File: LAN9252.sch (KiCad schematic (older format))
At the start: 52 parts, among them U1 LAN9252, U2 24LC00, Y1 Crystal_GND24

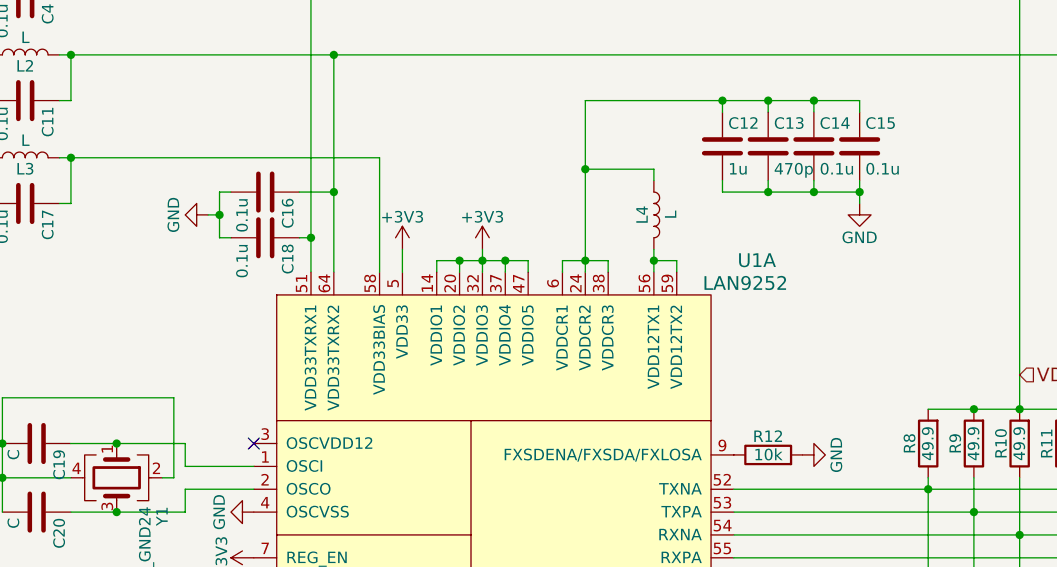
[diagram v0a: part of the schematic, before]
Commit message: 進捗
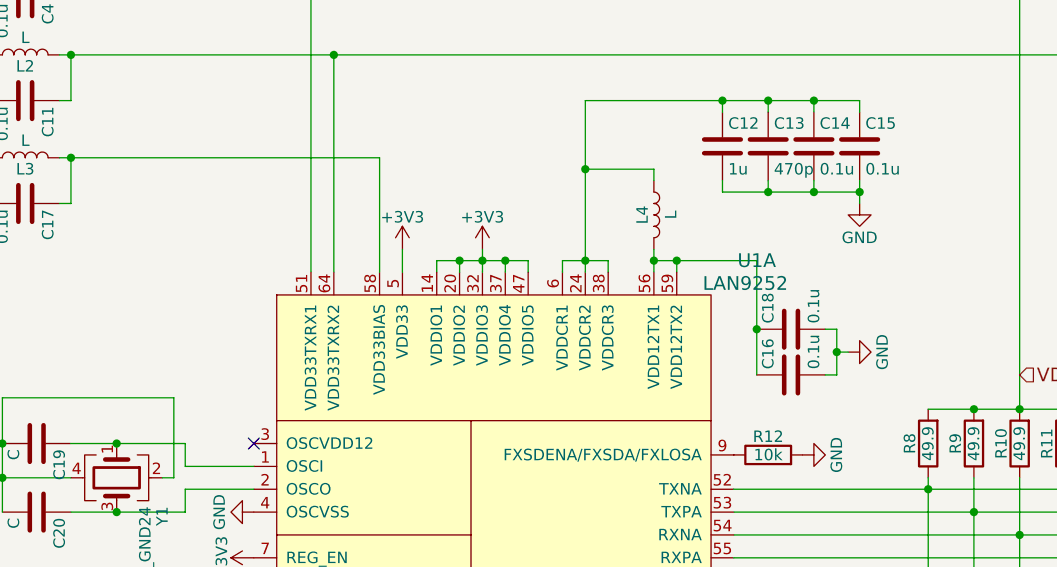
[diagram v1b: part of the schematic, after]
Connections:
- net VDD33TXRX1: no longer C18.1
- net VDDTXRX2: no longer C16.1
- net at L4.2, U1.56 (VDD12TX1), U1.59 (VDD12TX2): now also C16.1, C18.1
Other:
- moved on the sheet: C16, C18
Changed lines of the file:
@@
 $EndDescr
 $Comp
-L GND #PWR46
+L GND #PWR022
 U 1 1 58D8F4AE
 P 6400 6000
-F 0 "#PWR46" H 6400 5750 50  0001 C CNN
+F 0 "#PWR022" H 6400 5750 50  0001 C CNN
 F 1 "GND" H 6400 5850 50  0000 C CNN
 F 2 "" H 6400 6000 50  0000 C CNN
@@
 NoConn ~ 4600 3850
 $Comp
-L GND #PWR32
+L GND #PWR023
 U 1 1 58D8FBF8
 P 4600 4150
-F 0 "#PWR32" H 4600 3900 50  0001 C CNN
+F 0 "#PWR023" H 4600 3900 50  0001 C CNN
 F 1 "GND" H 4600 4000 50  0000 C CNN
 F 2 "" H 4600 4150 50  0000 C CNN
@@
 $EndComp
 $Comp
-L GND #PWR34
+L GND #PWR024
 U 1 1 58D8FC8D
 P 4250 4500
-F 0 "#PWR34" H 4250 4250 50  0001 C CNN
+F 0 "#PWR024" H 4250 4250 50  0001 C CNN
 F 1 "GND" H 4250 4350 50  0000 C CNN
 F 2 "" H 4250 4500 50  0000 C CNN
@@
 $EndComp
 $Comp
-L GND #PWR40
+L GND #PWR025
 U 1 1 58D8FD81
 P 4600 5100
-F 0 "#PWR40" H 4600 4850 50  0001 C CNN
+F 0 "#PWR025" H 4600 4850 50  0001 C CNN
 F 1 "GND" H 4600 4950 50  0000 C CNN
 F 2 "" H 4600 5100 50  0000 C CNN
@@
 $EndComp
 $Comp
-L GND #PWR30
+L GND #PWR026
 U 1 1 58D8CF70
 P 7000 3900
-F 0 "#PWR30" H 7000 3650 50  0001 C CNN
+F 0 "#PWR026" H 7000 3650 50  0001 C CNN
 F 1 "GND" H 7000 3750 50  0000 C CNN
 F 2 "" H 7000 3900 50  0000 C CNN
@@
 $EndComp
 $Comp
-L GND #PWR41
+L GND #PWR027
 U 1 1 58D8D10E
 P 7000 5350
-F 0 "#PWR41" H 7000 5100 50  0001 C CNN
+F 0 "#PWR027" H 7000 5100 50  0001 C CNN
 F 1 "GND" H 7000 5200 50  0000 C CNN
 F 2 "" H 7000 5350 50  0000 C CNN
@@
 $EndComp
 $Comp
-L GND #PWR35
+L GND #PWR028
 U 1 1 58D8D588
 P 8150 4700
-F 0 "#PWR35" H 8150 4450 50  0001 C CNN
+F 0 "#PWR028" H 8150 4450 50  0001 C CNN
 F 1 "GND" H 8150 4550 50  0000 C CNN
 F 2 "" H 8150 4700 50  0000 C CNN
@@
 $EndComp
 $Comp
-L GND #PWR42
+L GND #PWR029
 U 1 1 58D8F32E
 P 9350 5550
-F 0 "#PWR42" H 9350 5300 50  0001 C CNN
+F 0 "#PWR029" H 9350 5300 50  0001 C CNN
 F 1 "GND" H 9350 5400 50  0000 C CNN
 F 2 "" H 9350 5550 50  0000 C CNN
@@
 L C C18
 U 1 1 58DAEAFD
-P 4650 2950
-F 0 "C18" H 4675 3050 50  0000 L CNN
-F 1 "0.1u" H 4675 2850 50  0000 L CNN
-F 2 "Capacitors_SMD:C_0603" H 4688 2800 50  0001 C CNN
-F 3 "" H 4650 2950 50  0000 C CNN
-	1    4650 2950
-	0    1    1    0
+P 6950 3350
+F 0 "C18" H 6975 3450 50  0000 L CNN
+F 1 "0.1u" H 6975 3250 50  0000 L CNN
+F 2 "Capacitors_SMD:C_0603" H 6988 3200 50  0001 C CNN
+F 3 "" H 6950 3350 50  0000 C CNN
+	1    6950 3350
+	0    -1   -1   0
 $EndComp
 $Comp
 L C C16
 U 1 1 58DAEF7E
-P 4650 2750
-F 0 "C16" H 4675 2850 50  0000 L CNN
-F 1 "0.1u" H 4675 2650 50  0000 L CNN
-F 2 "Capacitors_SMD:C_0603" H 4688 2600 50  0001 C CNN
-F 3 "" H 4650 2750 50  0000 C CNN
-	1    4650 2750
-	0    1    1    0
-$EndComp
-$Comp
-L GND #PWR26
+P 6950 3550
+F 0 "C16" H 6975 3650 50  0000 L CNN
+F 1 "0.1u" H 6975 3450 50  0000 L CNN
+F 2 "Capacitors_SMD:C_0603" H 6988 3400 50  0001 C CNN
+F 3 "" H 6950 3550 50  0000 C CNN
+	1    6950 3550
+	0    -1   -1   0
+$EndComp
+$Comp
+L GND #PWR030
 U 1 1 58DAEFCA
-P 4400 2850
-F 0 "#PWR26" H 4400 2600 50  0001 C CNN
-F 1 "GND" H 4400 2700 50  0000 C CNN
-F 2 "" H 4400 2850 50  0000 C CNN
-F 3 "" H 4400 2850 50  0000 C CNN
-	1    4400 2850
-	0    1    1    0
+P 7200 3450
+F 0 "#PWR030" H 7200 3200 50  0001 C CNN
+F 1 "GND" H 7200 3300 50  0000 C CNN
+F 2 "" H 7200 3450 50  0000 C CNN
+F 3 "" H 7200 3450 50  0000 C CNN
+	1    7200 3450
+	0    -1   -1   0
 $EndComp
 $Comp
@@
 $EndComp
 $Comp
-L GND #PWR31
+L GND #PWR031
 U 1 1 58DB2B81
 P 3500 4000
-F 0 "#PWR31" H 3500 3750 50  0001 C CNN
+F 0 "#PWR031" H 3500 3750 50  0001 C CNN
 F 1 "GND" H 3500 3850 50  0000 C CNN
 F 2 "" H 3500 4000 50  0000 C CNN
@@
 $EndComp
 $Comp
-L +3V3 #PWR22
+L +3V3 #PWR032
 U 1 1 58DB404A
 P 3350 1600
-F 0 "#PWR22" H 3350 1450 50  0001 C CNN
+F 0 "#PWR032" H 3350 1450 50  0001 C CNN
 F 1 "+3V3" H 3350 1740 50  0000 C CNN
 F 2 "" H 3350 1600 50  0000 C CNN
@@
 $EndComp
 $Comp
-L GND #PWR27
+L GND #PWR033
 U 1 1 58DBACA0
 P 3400 3000
-F 0 "#PWR27" H 3400 2750 50  0001 C CNN
+F 0 "#PWR033" H 3400 2750 50  0001 C CNN
 F 1 "GND" H 3400 2850 50  0000 C CNN
 F 2 "" H 3400 3000 50  0000 C CNN
@@
 $EndComp
 $Comp
-L +3V3 #PWR28
+L +3V3 #PWR034
 U 1 1 58DBB1A4
 P 5250 3000
-F 0 "#PWR28" H 5250 2850 50  0001 C CNN
+F 0 "#PWR034" H 5250 2850 50  0001 C CNN
 F 1 "+3V3" H 5250 3140 50  0000 C CNN
 F 2 "" H 5250 3000 50  0000 C CNN
@@
 $EndComp
 $Comp
-L +3V3 #PWR29
+L +3V3 #PWR035
 U 1 1 58DBB719
 P 5600 3000
-F 0 "#PWR29" H 5600 2850 50  0001 C CNN
+F 0 "#PWR035" H 5600 2850 50  0001 C CNN
 F 1 "+3V3" H 5600 3140 50  0000 C CNN
 F 2 "" H 5600 3000 50  0000 C CNN
@@
 $EndComp
 $Comp
-L +3V3 #PWR33
+L +3V3 #PWR036
 U 1 1 58DBBE53
 P 4600 4350
-F 0 "#PWR33" H 4600 4200 50  0001 C CNN
+F 0 "#PWR036" H 4600 4200 50  0001 C CNN
 F 1 "+3V3" H 4600 4490 50  0000 C CNN
 F 2 "" H 4600 4350 50  0000 C CNN
@@
 $EndComp
 $Comp
-L GND #PWR25
+L GND #PWR037
 U 1 1 58DBE707
 P 7250 2800
-F 0 "#PWR25" H 7250 2550 50  0001 C CNN
+F 0 "#PWR037" H 7250 2550 50  0001 C CNN
 F 1 "GND" H 7250 2650 50  0000 C CNN
 F 2 "" H 7250 2800 50  0000 C CNN
@@
 $EndComp
 $Comp
-L GND #PWR24
+L GND #PWR038
 U 1 1 58DC454A
 P 2300 2450
-F 0 "#PWR24" H 2300 2200 50  0001 C CNN
+F 0 "#PWR038" H 2300 2200 50  0001 C CNN
 F 1 "GND" H 2300 2300 50  0000 C CNN
 F 2 "" H 2300 2450 50  0000 C CNN
@@
 $EndComp
 $Comp
-L +3V3 #PWR23
+L +3V3 #PWR039
 U 1 1 58DC4AF2
 P 2300 1950
-F 0 "#PWR23" H 2300 1800 50  0001 C CNN
+F 0 "#PWR039" H 2300 1800 50  0001 C CNN
 F 1 "+3V3" H 2300 2090 50  0000 C CNN
 F 2 "" H 2300 1950 50  0000 C CNN
@@
 $EndComp
 $Comp
-L +3V3 #PWR44
+L +3V3 #PWR040
 U 1 1 58DC9090
 P 3150 5800
-F 0 "#PWR44" H 3150 5650 50  0001 C CNN
+F 0 "#PWR040" H 3150 5650 50  0001 C CNN
 F 1 "+3V3" H 3150 5940 50  0000 C CNN
 F 2 "" H 3150 5800 50  0000 C CNN
@@
 $EndComp
 $Comp
-L GND #PWR47
+L GND #PWR041
 U 1 1 58DCCAA2
 P 4450 6300
-F 0 "#PWR47" H 4450 6050 50  0001 C CNN
+F 0 "#PWR041" H 4450 6050 50  0001 C CNN
 F 1 "GND" H 4450 6150 50  0000 C CNN
 F 2 "" H 4450 6300 50  0000 C CNN
@@
 $EndComp
 $Comp
-L GND #PWR39
+L GND #PWR042
 U 1 1 58DD07AD
 P 4250 4950
-F 0 "#PWR39" H 4250 4700 50  0001 C CNN
+F 0 "#PWR042" H 4250 4700 50  0001 C CNN
 F 1 "GND" H 4250 4800 50  0000 C CNN
 F 2 "" H 4250 4950 50  0000 C CNN
@@
 $EndComp
 $Comp
-L +3V3 #PWR38
+L +3V3 #PWR043
 U 1 1 58DD57EA
 P 3650 4850
-F 0 "#PWR38" H 3650 4700 50  0001 C CNN
+F 0 "#PWR043" H 3650 4700 50  0001 C CNN
 F 1 "+3V3" H 3650 4990 50  0000 C CNN
 F 2 "" H 3650 4850 50  0000 C CNN
@@
 	6350 3000 6350 3100
 Wire Wire Line
-	6350 3050 6450 3050
+	6350 3050 6800 3050
 Wire Wire Line
 	6450 3050 6450 3100
@@
 	4950 2150 4950 3100
 Wire Wire Line
-	4800 2950 4850 2950
-Connection ~ 4850 2950
-Wire Wire Line
-	4800 2750 4950 2750
-Connection ~ 4950 2750
-Wire Wire Line
-	4450 2950 4500 2950
-Wire Wire Line
-	4450 2750 4450 2950
-Wire Wire Line
-	4450 2750 4500 2750
-Wire Wire Line
-	4400 2850 4450 2850
-Connection ~ 4450 2850
+	7150 3350 7100 3350
+Wire Wire Line
+	7150 3550 7150 3350
+Wire Wire Line
+	7150 3550 7100 3550
+Wire Wire Line
+	7200 3450 7150 3450
+Connection ~ 7150 3450
 Wire Wire Line
 	3500 3650 3500 4150
@@
 	3000 5200 3000 5400
 $Comp
-L GND #PWR43
+L GND #PWR044
 U 1 1 58E26D3D
 P 2150 5600
-F 0 "#PWR43" H 2150 5350 50  0001 C CNN
+F 0 "#PWR044" H 2150 5350 50  0001 C CNN
 F 1 "GND" H 2150 5450 50  0000 C CNN
 F 2 "" H 2150 5600 50  0000 C CNN
@@
 Connection ~ 1700 5300
 $Comp
-L GND #PWR45
+L GND #PWR045
 U 1 1 58E27E20
 P 1700 5900
-F 0 "#PWR45" H 1700 5650 50  0001 C CNN
+F 0 "#PWR045" H 1700 5650 50  0001 C CNN
 F 1 "GND" H 1700 5750 50  0000 C CNN
 F 2 "" H 1700 5900 50  0000 C CNN
@@
 $EndComp
 $Comp
-L GND #PWR37
+L GND #PWR046
 U 1 1 58E29423
 P 1750 4850
-F 0 "#PWR37" H 1750 4600 50  0001 C CNN
+F 0 "#PWR046" H 1750 4600 50  0001 C CNN
 F 1 "GND" H 1750 4700 50  0000 C CNN
 F 2 "" H 1750 4850 50  0000 C CNN
@@
 $EndComp
 $Comp
-L +3V3 #PWR36
+L +3V3 #PWR047
 U 1 1 58E2970F
 P 2150 4750
-F 0 "#PWR36" H 2150 4600 50  0001 C CNN
+F 0 "#PWR047" H 2150 4600 50  0001 C CNN
 F 1 "+3V3" H 2150 4890 50  0000 C CNN
 F 2 "" H 2150 4750 50  0000 C CNN
@@
 	1    0    0    -1
 $EndComp
+Wire Wire Line
+	6800 3050 6800 3550
+Connection ~ 6450 3050
+Connection ~ 6800 3350
 $EndSCHEMATC
